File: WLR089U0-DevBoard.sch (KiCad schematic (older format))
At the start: 23 parts, among them IC1 WLR089U0-I_RM, J1 USB_B_Micro, J2 Conn_01x10_Female, J3 Conn_01x10_Female, J3 Conn_ARM_JTAG_SWD_10, J6 Conn_01x04_Male, J8 Conn_01x06_Male, SW1 SW_Push, U1 MCP1700-3302E_SOT23, U4 CH304e

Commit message: Beautified schematic layout, ERC pending
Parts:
- removed J6: Conn_01x04_Male, symbol Connector:Conn_01x04_Male
- removed JP3, JP4, JP5: SolderJumper_2_Bridged, symbol Jumper:SolderJumper_2_Bridged
- removed U4: CH304e, symbol Interface_USB:CH304e
- added JP3: SolderJumper_2_Open, symbol Jumper:SolderJumper_2_Open
- added U2: CH304E, symbol WLR089U0-DevBoard-rescue:CH304E
- J4: renamed from J8; value Conn_01x06_Male -> Conn_01x10_Male; symbol Connector:Conn_01x06_Male -> Connector:Conn_01x10_Male
- renumbered C4 to C3, J3 to J2, J2 to J3, J3 to J5, JP2 to JP1, JP1 to JP2, R2 to R1, R1 to R2
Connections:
- net labels removed: SWCLK
- wire segments 109 -> 114
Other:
- note added: "ARM CORTEX SWD PROGRAMMING\n10 PIN HEADER"
- note added: "BLANK SPACE"
- note added: "GPIO PIN HEADERS"
- note added: "GPIO STATUS LED"
- note added: "I2C & SPI HEADER"
- note added: "Microchip WLR089U0-SAMR34 Module"
- note added: "POWER CIRCUITRY"
- note added: "POWER LED"
- note added: "USB-UART USING CH340E via JP3 short (OR)\nUSB-USB via JP1,JP2 short"
- note removed: "POWER CURCUITRY"
- note removed: "Programming unit"
- note removed: "WLR089U0-SAMR34-Dev-Board-LoRaWAN"
- moved on the sheet: C1, C2, C3, D1, D2, IC1, J1, J2, J3, J5, JP1, JP2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

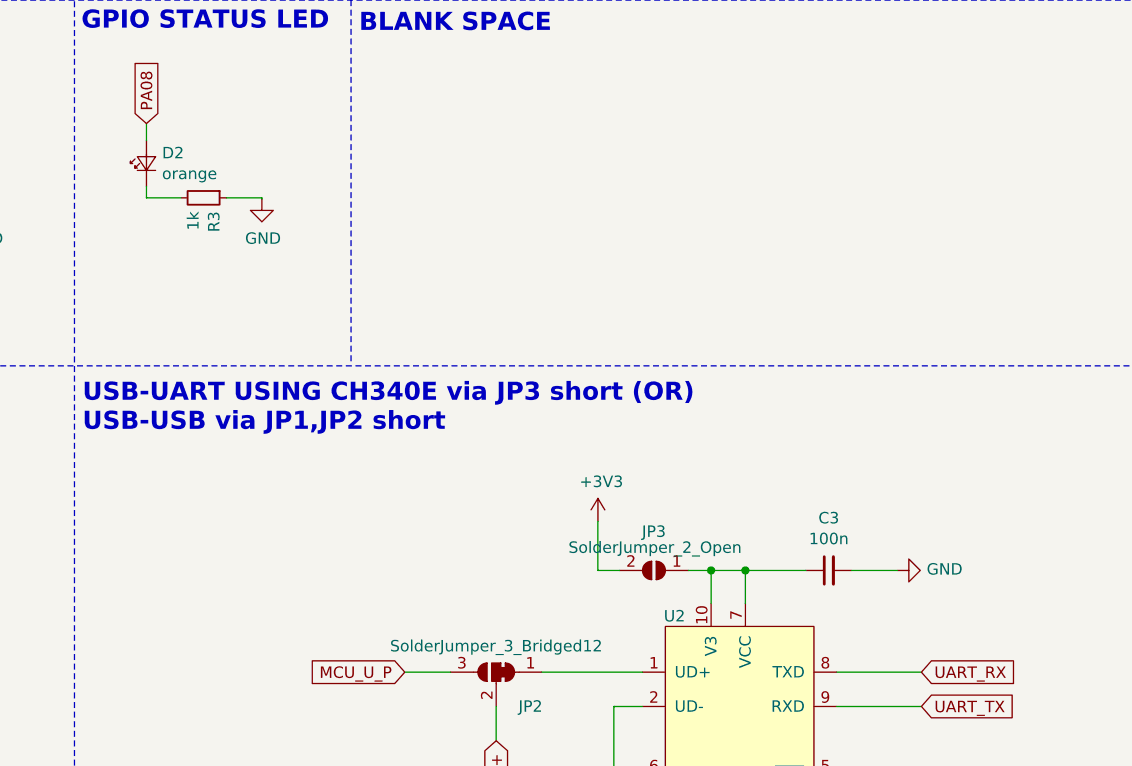
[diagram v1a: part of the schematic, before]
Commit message: final schematic
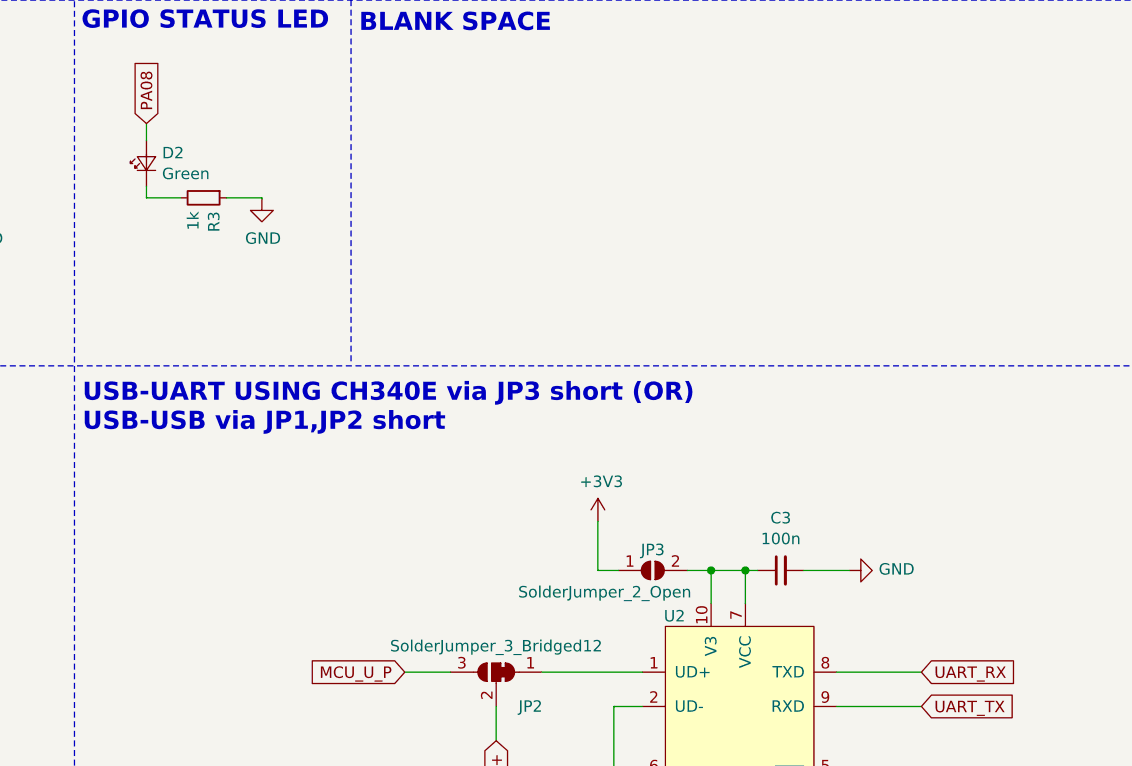
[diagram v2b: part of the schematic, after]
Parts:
- D2: value orange -> Green
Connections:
- net +3V3: now also JP3.1 (A); no longer JP3.2 (B)
- net at C3.1, U2.10 (V3), U2.7 (VCC): now also JP3.2 (B); no longer JP3.1 (A)
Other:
- moved on the sheet: C3
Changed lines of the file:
@@
 EESchema Schematic File Version 4
+LIBS:WLR089U0-DevBoard-cache
 EELAYER 30 0
 EELAYER END
@@
 P 6350 1265
 F 0 "D2" V 6396 1197 50  0000 R CNN
-F 1 "orange " V 6305 1197 50  0000 R CNN
+F 1 "Green" V 6305 1197 50  0000 R CNN
 F 2 "" V 6350 1265 50  0001 C CNN
 F 3 "~" V 6350 1265 50  0001 C CNN
@@
 L Device:C_Small C3
 U 1 1 602D3CA5
-P 9335 3045
-F 0 "C3" V 9564 3045 50  0000 C CNN
-F 1 "100n" V 9473 3045 50  0000 C CNN
-F 2 "" H 9335 3045 50  0001 C CNN
-F 3 "~" H 9335 3045 50  0001 C CNN
-	1    9335 3045
+P 9125 3045
+F 0 "C3" V 9354 3045 50  0000 C CNN
+F 1 "100n" V 9263 3045 50  0000 C CNN
+F 2 "" H 9125 3045 50  0001 C CNN
+F 3 "~" H 9125 3045 50  0001 C CNN
+	1    9125 3045
 	0    -1   -1   0
 $EndComp
@@
 L power:GND #PWR022
 U 1 1 602D61C1
-P 9635 3045
-F 0 "#PWR022" H 9635 2795 50  0001 C CNN
-F 1 "GND" V 9640 2917 50  0000 R CNN
-F 2 "" H 9635 3045 50  0001 C CNN
-F 3 "" H 9635 3045 50  0001 C CNN
-	1    9635 3045
+P 9425 3045
+F 0 "#PWR022" H 9425 2795 50  0001 C CNN
+F 1 "GND" V 9430 2917 50  0000 R CNN
+F 2 "" H 9425 3045 50  0001 C CNN
+F 3 "" H 9425 3045 50  0001 C CNN
+	1    9425 3045
 	0    -1   -1   0
 $EndComp
 Wire Wire Line
-	9435 3045 9635 3045
+	9225 3045 9425 3045
 $Comp
 L Regulator_Linear:MCP1700-3302E_SOT23 U1
@@
 	1    0    0    -1
 $EndComp
-Wire Wire Line
-	8820 3045 8970 3045
-Connection ~ 8970 3045
 Text Notes 570  5465 0    79   ~ 16
 ARM CORTEX SWD PROGRAMMING\n10 PIN HEADER
@@
 	1650 7260 1600 7260
 Connection ~ 1600 7260
-Wire Wire Line
-	8970 3045 9235 3045
 Text GLabel 9740 3640 2    50   Input ~ 0
 UART_TX
@@
 Wire Wire Line
 	8075 4175 8395 4175
-$Comp
-L Jumper:SolderJumper_2_Open JP3
-U 1 1 6031D154
-P 8570 3045
-F 0 "JP3" H 8570 2875 50  0000 C CNN
-F 1 "SolderJumper_2_Open" H 8565 2945 50  0000 C CNN
-F 2 "" H 8570 3045 50  0001 C CNN
-F 3 "~" H 8570 3045 50  0001 C CNN
-	1    8570 3045
-	-1   0    0    1
-$EndComp
-Wire Wire Line
-	8720 3045 8820 3045
 Connection ~ 8820 3045
 Wire Wire Line
 	8325 2830 8325 3045
-Wire Wire Line
-	8325 3045 8420 3045
 Text Notes 6950 5340 0    79   ~ 16
 I2C & SPI HEADER
@@
 Text GLabel 4255 6190 0    50   Input ~ 0
 PA07
+$Comp
+L Jumper:SolderJumper_2_Open JP3
+U 1 1 601C47FE
+P 8565 3045
+F 0 "JP3" H 8565 3135 50  0000 C CNN
+F 1 "SolderJumper_2_Open" H 8355 2950 50  0000 C CNN
+F 2 "" H 8565 3045 50  0001 C CNN
+F 3 "~" H 8565 3045 50  0001 C CNN
+	1    8565 3045
+	1    0    0    -1
+$EndComp
+Wire Wire Line
+	8715 3045 8820 3045
+Wire Wire Line
+	8325 3045 8415 3045
+Wire Wire Line
+	8820 3045 8970 3045
+Connection ~ 8970 3045
+Wire Wire Line
+	8970 3045 9025 3045
 $EndSCHEMATC
